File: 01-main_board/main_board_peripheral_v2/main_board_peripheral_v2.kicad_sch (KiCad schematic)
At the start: 19 parts, among them J2 T4040014041000, J3 T4041017041-000, J4 DF12NB_5.0_-20DP-0.5V_51_, Q1 SSF2302, U1 LM74610QDGKRQ1, U2 TPS613222ADBVR

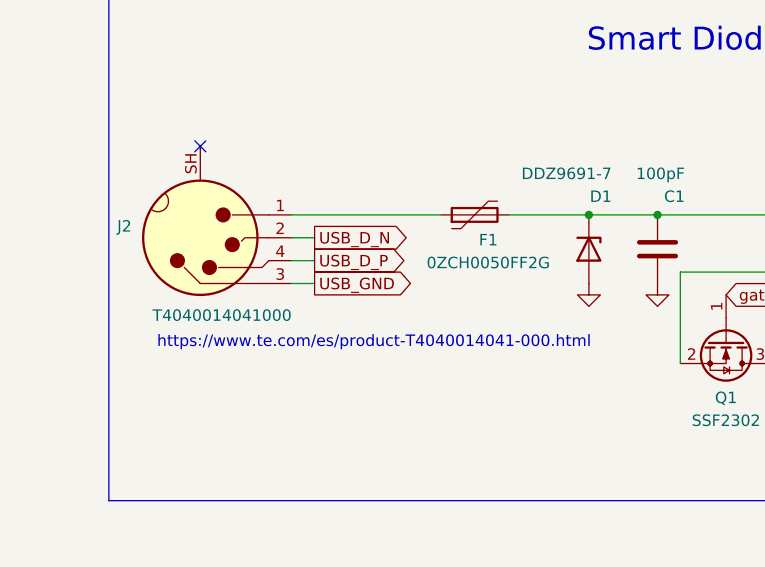
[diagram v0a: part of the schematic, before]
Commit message: layout done
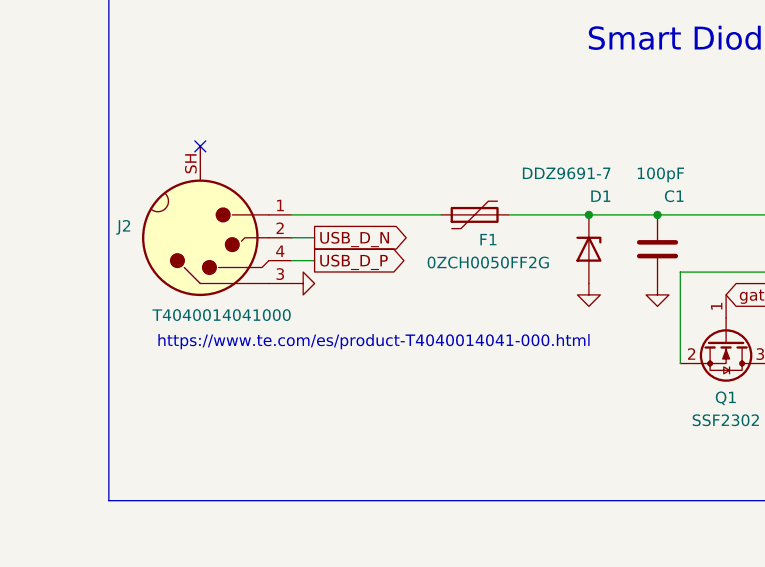
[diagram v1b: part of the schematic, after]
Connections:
- net USB_GND is gone; now on net GND: J2.3
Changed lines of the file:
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@@
 	(wire
 		(pts
-			(xy 39.37 52.07) (xy 41.91 52.07)
+			(xy 82.55 50.8) (xy 82.55 60.96)
 		)
 		(stroke
@@
 		)
 	)
-	(wire
+	(bus
 		(pts
-			(xy 82.55 50.8) (xy 82.55 60.96)
+			(xy 180.34 19.05) (xy 19.05 19.05)
 		)
 		(stroke
@@
 	(bus
 		(pts
-			(xy 180.34 19.05) (xy 19.05 19.05)
+			(xy 180.34 19.05) (xy 180.34 76.2)
 		)
 		(stroke
@@
 		)
 	)
-	(bus
+	(wire
 		(pts
-			(xy 180.34 19.05) (xy 180.34 76.2)
+			(xy 160.02 34.29) (xy 166.37 34.29)
 		)
 		(stroke
@@
 	(wire
 		(pts
-			(xy 160.02 34.29) (xy 166.37 34.29)
+			(xy 104.14 46.99) (xy 96.52 46.99)
 		)
 		(stroke
@@
 		)
 	)
-	(wire
+	(bus
 		(pts
-			(xy 104.14 46.99) (xy 96.52 46.99)
+			(xy 19.05 76.2) (xy 180.34 76.2)
 		)
 		(stroke
@@
 		)
 	)
-	(bus
+	(wire
 		(pts
-			(xy 19.05 76.2) (xy 180.34 76.2)
+			(xy 96.52 60.96) (xy 92.71 60.96)
 		)
 		(stroke
@@
 		)
 	)
-	(wire
+	(bus
 		(pts
-			(xy 96.52 60.96) (xy 92.71 60.96)
+			(xy 19.05 19.05) (xy 19.05 76.2)
 		)
 		(stroke
@@
 		)
 	)
-	(bus
+	(wire
 		(pts
-			(xy 19.05 19.05) (xy 19.05 76.2)
+			(xy 96.52 64.77) (xy 102.87 64.77)
 		)
 		(stroke
@@
 	(wire
 		(pts
-			(xy 96.52 64.77) (xy 102.87 64.77)
+			(xy 63.5 44.45) (xy 72.39 44.45)
 		)
 		(stroke
@@
 	(wire
 		(pts
-			(xy 63.5 44.45) (xy 72.39 44.45)
+			(xy 256.54 63.5) (xy 250.19 63.5)
 		)
 		(stroke
@@
 	(wire
 		(pts
-			(xy 256.54 63.5) (xy 250.19 63.5)
+			(xy 160.02 36.83) (xy 160.02 34.29)
 		)
 		(stroke
@@
 		)
 	)
-	(wire
-		(pts
-			(xy 160.02 36.83) (xy 160.02 34.29)
-		)
-		(stroke
-			(width 0)
-			(type default)
-		)
-	)
 	(global_label "RX_P"
 		(shape bidirectional)
@@
 		(property "Intersheetrefs" "${INTERSHEET_REFS}"
 			(at 97.0425 52.07 0)
-			(effects
-				(font
-					(size 1.27 1.27)
-				)
-				(justify right)
-				(hide yes)
-			)
-		)
-	)
-	(global_label "USB_GND"
-		(shape output)
-		(at 41.91 52.07 0)
-		(fields_autoplaced yes)
-		(effects
-			(font
-				(size 1.27 1.27)
-			)
-			(justify left)
-		)
-		(property "Intersheetrefs" "${INTERSHEET_REFS}"
-			(at 30.2767 52.07 0)
 			(effects
 				(font
@@
 					(unit 1)
 				)
+			)
+		)
+	)
+	(symbol
+		(lib_id "power:GND")
+		(at 39.37 52.07 90)
+		(unit 1)
+		(exclude_from_sim no)
+		(in_bom yes)
+		(on_board yes)
+		(dnp no)
+		(fields_autoplaced yes)
+		(property "Reference" "#PWR01"
+			(at 45.72 52.07 0)
+			(effects
+				(font
+					(size 1.27 1.27)
+				)
+				(hide yes)
+			)
+		)
+		(property "Value" "GND"
+			(at 44.45 52.07 0)
+			(effects
+				(font
+					(size 1.27 1.27)
+				)
+				(hide yes)
+			)
+		)
+		(property "Footprint" ""
+			(at 39.37 52.07 0)
+			(effects
+				(font
+					(size 1.27 1.27)
+				)
+				(hide yes)
+			)
+		)
+		(property "Datasheet" ""
+			(at 39.37 52.07 0)
+			(effects
+				(font
+					(size 1.27 1.27)
+				)
+				(hide yes)
+			)
+		)
+		(property "Description" "Power symbol creates a global label with name \"GND\" , ground"
+			(at 39.37 52.07 0)
+			(effects
+				(font
+					(size 1.27 1.27)
+				)
+				(hide yes)
+			)
+		)
+		(pin "1"
+		)
+		(instances
+			(project "main_board_peripheral_v2"
+				(path "/3f673207-cdae-494a-ab60-6e58b06fb202"
+					(reference "#PWR01")
+					(unit 1)
+				)

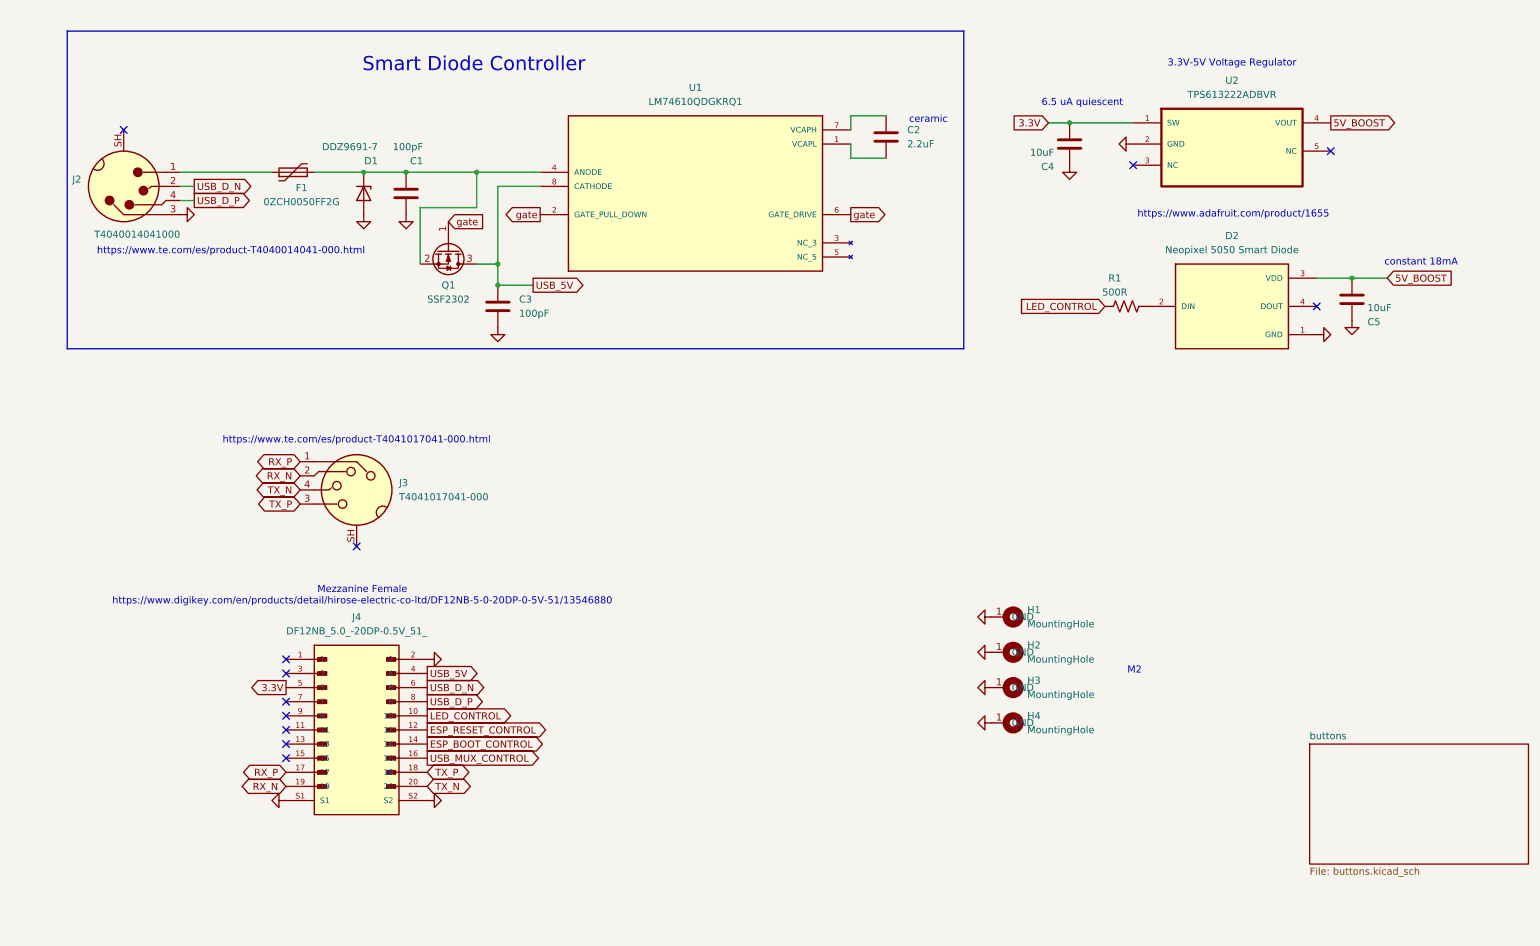
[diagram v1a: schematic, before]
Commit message: Push to change computers. New schematic.
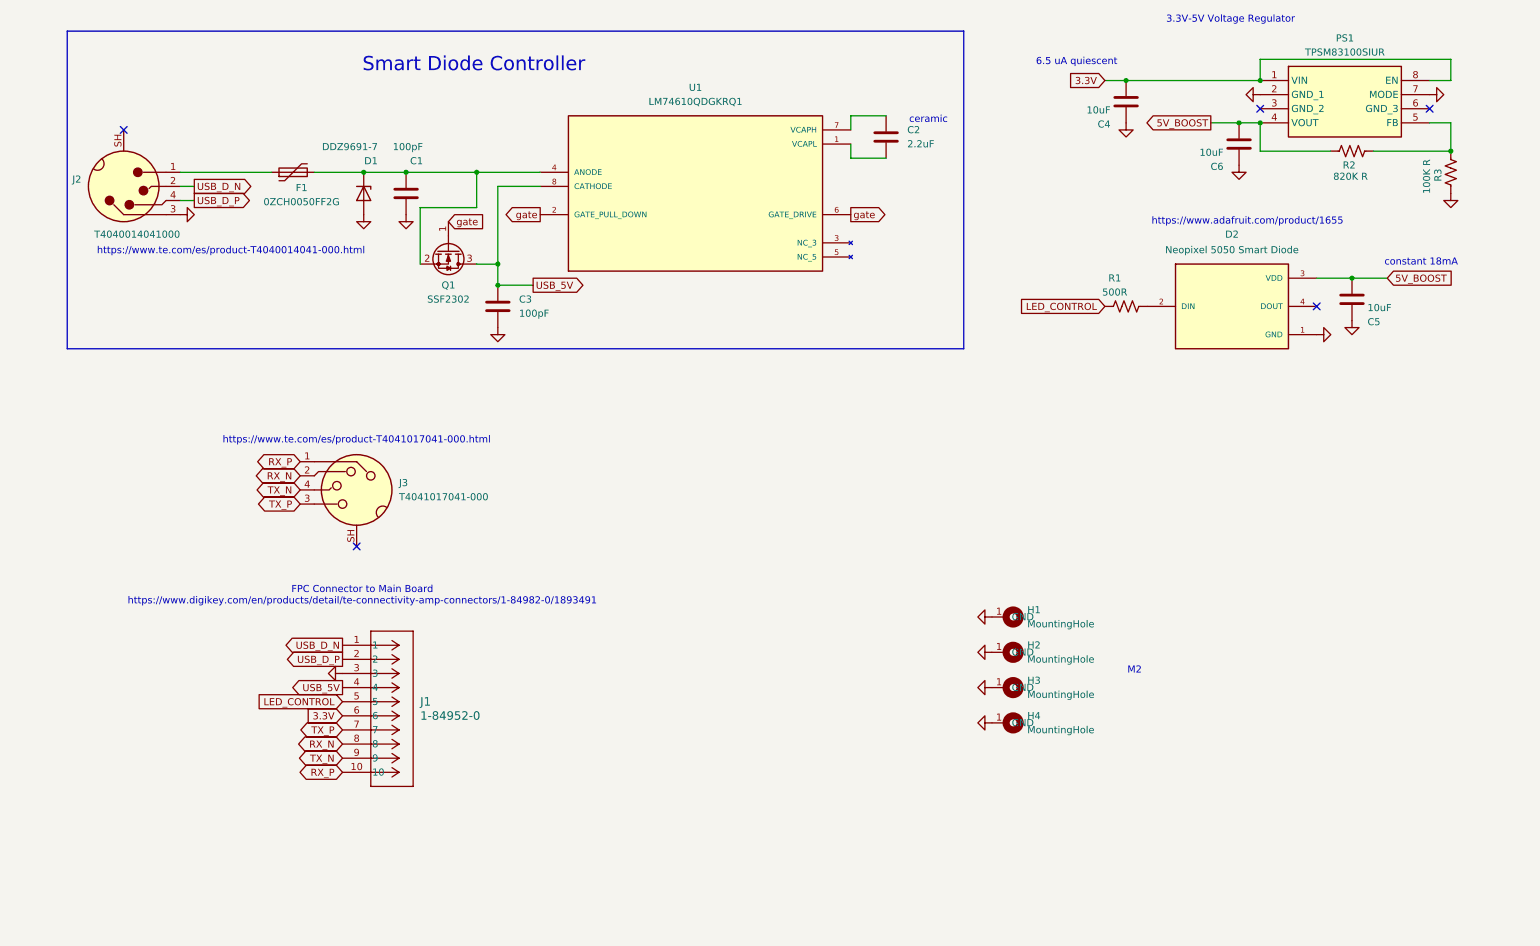
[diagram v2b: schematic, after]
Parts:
- removed J4: DF12NB_5.0_-20DP-0.5V_51_, 22XT_Main_Peripheral:DF12NB_5.0_-20DP-0.5V_51_, symbol DF12NB_5.0_-20DP-0.5V_51_:DF12NB_5.0_-20DP-0.5V_51_
- removed U2: TPS613222ADBVR, 22XT_Main_Peripheral:TPS613222ADBVR, symbol TPS613222ADBVR:TPS613222ADBVR
- added C6: 10uF, Capacitor_SMD:C_0603_1608Metric, symbol Device:C
- added J1: 1-84952-0, CONN10_1-84982-0_TEC, symbol 2026-02-06_01-22-38:1-84982-0
- added PS1: TPSM83100SIUR, TPSM83100SIUR, symbol 2026-02-06_01-22-38:TPSM83100SIUR
- added R2: 820K R, symbol Device:R_US
- added R3: 100K R, symbol Device:R_US
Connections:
- net 3.3V: now also J1.6, PS1.1 (VIN), PS1.8 (EN)
- net 5V_BOOST: now also C6.1, PS1.4 (VOUT), R2.2
- net GND: now also C6.2, J1.3, PS1.2 (GND_1), PS1.7 (MODE), R3.1
- net LED_CONTROL: now also J1.5
- net RX_N: now also J1.8
- net RX_P: now also J1.10
- net TX_N: now also J1.9
- net TX_P: now also J1.7
- net USB_5V: now also J1.4
- net USB_D_N: now also J1.1
- net USB_D_P: now also J1.2
- new net: PS1.5 (FB), R2.1, R3.2
- no-connect marks 12 -> 5
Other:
- removed sheet buttons
- note added: "FPC Connector to Main Board https://www.digikey.com/en/products/detail/te-connectivity-amp-connectors/1-84982-0/1893491"
- note removed: "Mezzanine Female https://www.digikey.com/en/products/detail/hirose-electric-co-ltd/DF12NB-5-0-20DP-0-5V-51/13546880"
- moved on the sheet: C4

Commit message: Started on layout
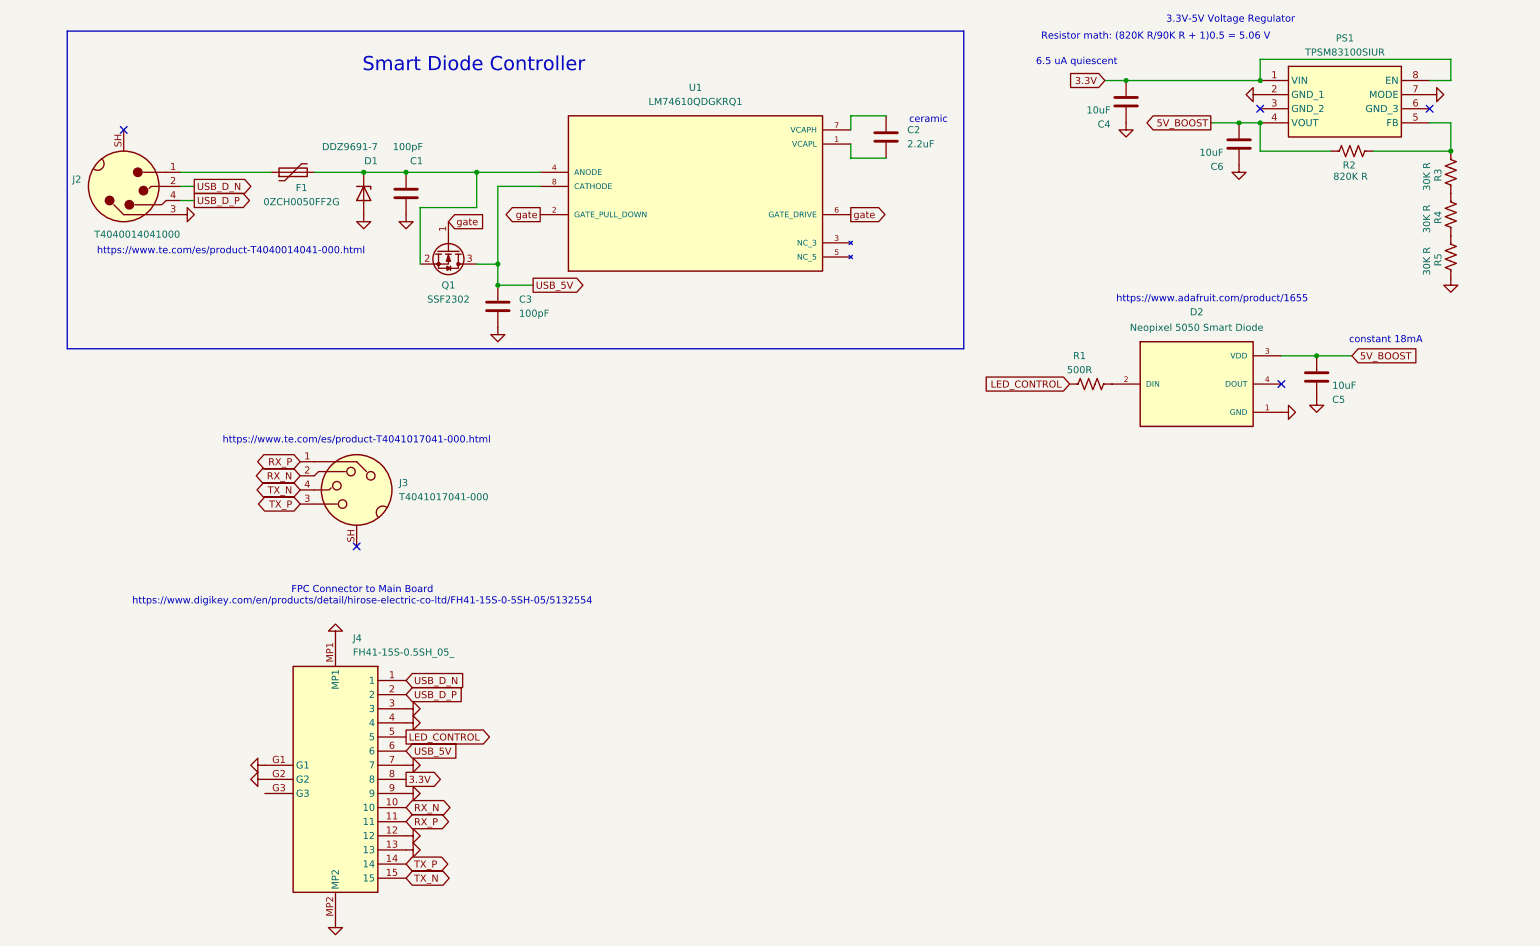
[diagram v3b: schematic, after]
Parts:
- removed H1, H2, H3, H4: MountingHole, MountingHole:MountingHole_2.2mm_M2_Pad, symbol Mechanical:MountingHole
- removed J1: 1-84952-0, CONN10_1-84982-0_TEC, symbol 2026-02-06_01-22-38:1-84982-0
- added J4: FH41-15S-0.5SH_05_, 22XT_Main_Peripheral:FH4115S05SH05, symbol FH41-15S-0_5SH_05_:FH41-15S-0.5SH_05_
- added R4, R5: 30K R, 22XT_Main_Peripheral:RESC3116X65N (30K), symbol Device:R_US
- PS1: footprint TPSM83100SIUR -> 22XT_Main_Peripheral:TPSM83100SIUR
- R2: footprint (none) -> 22XT_Main_Peripheral:RESC3116X65N (820K)
- R3: value 100K R -> 30K R; footprint (none) -> 22XT_Main_Peripheral:RESC3116X65N (30K)
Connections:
- net 3.3V: now also J4.8
- net GND: now also J4.12, J4.13, J4.3, J4.4, J4.7, J4.9, J4.G1, J4.G2, J4.MP1, J4.MP2, R5.1; no longer R3.1
- net LED_CONTROL: now also J4.5
- net RX_N: now also J4.10
- net RX_P: now also J4.11
- net TX_N: now also J4.15
- net TX_P: now also J4.14
- net USB_5V: now also J4.6
- net USB_D_N: now also J4.1
- net USB_D_P: now also J4.2
- new net: R4.1, R5.2
- new net: R3.1, R4.2
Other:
- note added: "FPC Connector to Main Board https://www.digikey.com/en/products/detail/hirose-electric-co-ltd/FH41-15S-0-5SH-05/5132554"
- note added: "Resistor math: (820K R/90K R + 1)0.5 = 5.06 V"
- note removed: "FPC Connector to Main Board https://www.digikey.com/en/products/detail/te-connectivity-amp-connectors/1-84982-0/1893491"
- note removed: "M2"
- moved on the sheet: C5, D2, R1
